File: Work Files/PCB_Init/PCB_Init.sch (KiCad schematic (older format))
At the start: 33 parts, among them J1 Conn_01x02_Female, J2 Screw_Terminal_01x02, J3 Conn_01x02_Female, J4 Conn_01x02_Female, J5 Conn_01x02_Female, J6 Conn_01x02_Female, J7 Conn_01x02_Female, SW1 SW_Push, SW2 SW_Push, SW3 SW_Push, SW4 SW_Push, U1 L7805, U2 NHD-0420H1Z, U3 40PC015G

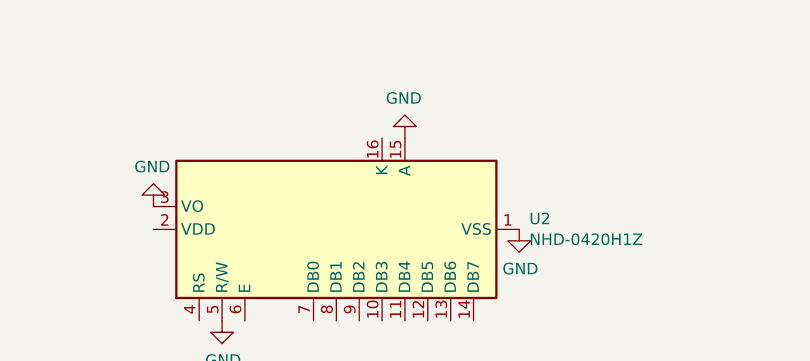
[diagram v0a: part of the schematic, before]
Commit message: Plotted gerber files for initial idea3
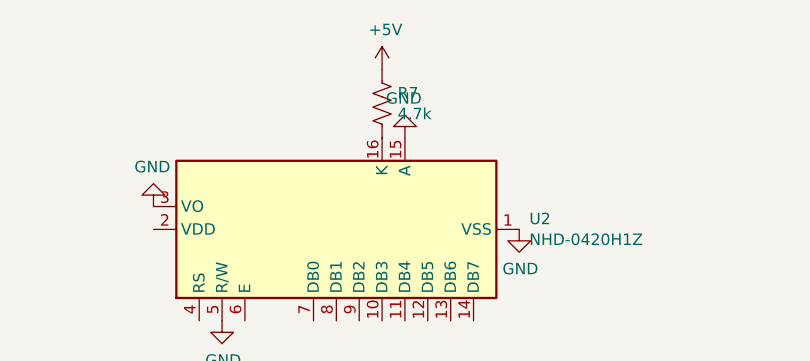
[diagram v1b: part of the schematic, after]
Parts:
- added R7: 4.7k, Resistor_THT:R_Axial_DIN0204_L3.6mm_D1.6mm_P5.08mm_Horizontal, symbol Device:R_US
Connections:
- net +5V: now also R7.1
- net at U2.16 (K): now also R7.2
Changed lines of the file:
@@
 Wire Wire Line
 	3150 4550 3150 4750
+$Comp
+L Device:R_US R7
+U 1 1 607FE3A9
+P 5350 900
+F 0 "R7" H 5418 946 50  0000 L CNN
+F 1 "4.7k" H 5418 855 50  0000 L CNN
+F 2 "Resistor_THT:R_Axial_DIN0204_L3.6mm_D1.6mm_P5.08mm_Horizontal" V 5390 890 50  0001 C CNN
+F 3 "~" H 5350 900 50  0001 C CNN
+F 4 "R" H 5350 900 50  0001 C CNN "Spice_Primitive"
+F 5 "4.7k" H 5350 900 50  0001 C CNN "Spice_Model"
+F 6 "Y" H 5350 900 50  0001 C CNN "Spice_Netlist_Enabled"
+	1    5350 900
+	1    0    0    -1
+$EndComp
+$Comp
+L power:+5V #PWR034
+U 1 1 607FEDA5
+P 5350 750
+F 0 "#PWR034" H 5350 600 50  0001 C CNN
+F 1 "+5V" H 5365 923 50  0000 C CNN
+F 2 "" H 5350 750 50  0001 C CNN
+F 3 "" H 5350 750 50  0001 C CNN
+	1    5350 750
+	1    0    0    -1
+$EndComp
 $EndSCHEMATC
